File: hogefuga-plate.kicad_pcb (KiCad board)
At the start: 2 copper layers, 95.2 x 76.2 mm, 23 parts

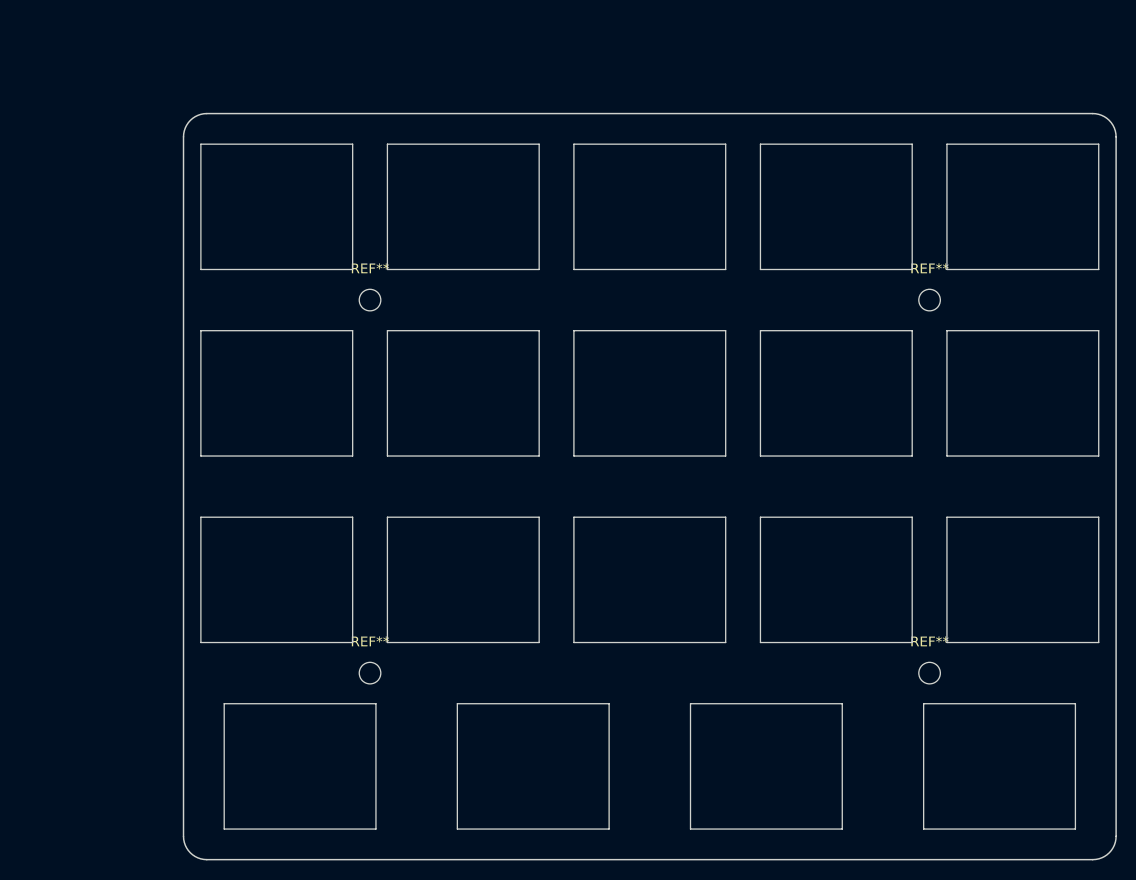
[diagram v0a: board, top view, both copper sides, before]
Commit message: rev0.2
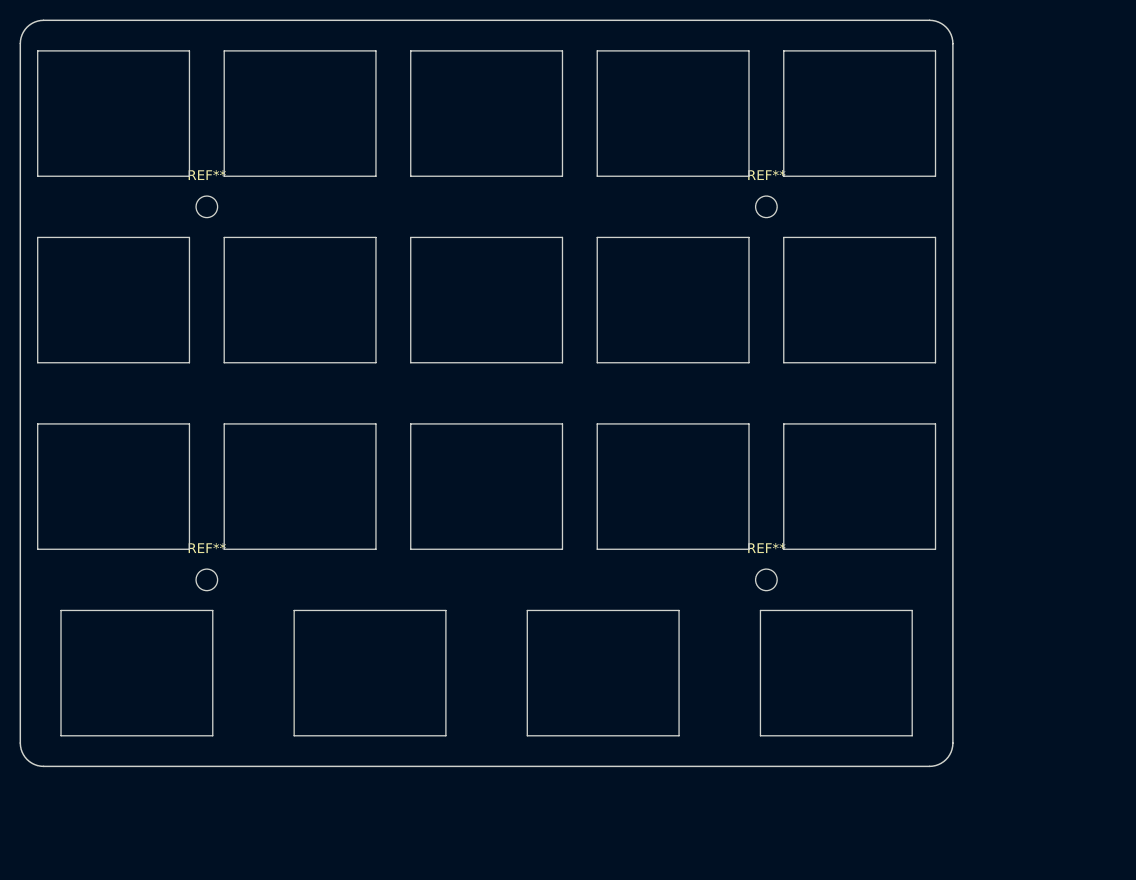
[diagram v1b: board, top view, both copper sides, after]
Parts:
- removed the ALPS_SKCM_CUTOUT at (119.1, 78.6)
- removed the ALPS_SKCM_CUTOUT at (157.2, 116.7)
- removed the ALPS_SKCM_CUTOUT at (81.0, 97.6)
- removed the ALPS_SKCM_CUTOUT at (154.8, 135.7)
- removed the ALPS_SKCM_CUTOUT at (107.2, 135.7)
- removed the ALPS_SKCM_CUTOUT at (138.1, 116.7)
- removed the ALPS_SKCM_CUTOUT at (81.0, 78.6)
- removed the ALPS_SKCM_CUTOUT at (119.1, 116.7)
- removed the ALPS_SKCM_CUTOUT at (81.0, 116.7)
- removed the ALPS_SKCM_CUTOUT at (157.2, 97.6)
- removed the ALPS_SKCM_CUTOUT at (119.1, 97.6)
- removed the ALPS_SKCM_CUTOUT at (100.0, 97.6)
- removed the ALPS_SKCM_CUTOUT at (100.0, 116.7)
- removed the ALPS_SKCM_CUTOUT at (157.2, 78.6)
- removed the ALPS_SKCM_CUTOUT at (131.0, 135.7)
- removed the ALPS_SKCM_CUTOUT at (83.3, 135.7)
- removed the ALPS_SKCM_CUTOUT at (138.1, 78.6)
- removed the ALPS_SKCM_CUTOUT at (100.0, 78.6)
- removed the ALPS_SKCM_CUTOUT at (138.1, 97.6)
- removed the REF** at (90.5, 126.2)
- removed the REF** at (147.6, 88.1)
- removed the REF** at (90.5, 88.1)
- removed the REF** at (147.6, 126.2)
- added ALPS_SKCM_CUTOUT: VAL**, keyboard_parts:ALPS_SKCM_CUTOUT, F.Cu at (140.5, 69.1)
- added ALPS_SKCM_CUTOUT: VAL**, keyboard_parts:ALPS_SKCM_CUTOUT, F.Cu at (64.3, 88.1)
- added ALPS_SKCM_CUTOUT: VAL**, keyboard_parts:ALPS_SKCM_CUTOUT, F.Cu at (64.3, 107.2)
- added ALPS_SKCM_CUTOUT: VAL**, keyboard_parts:ALPS_SKCM_CUTOUT, F.Cu at (83.3, 107.2)
- added ALPS_SKCM_CUTOUT: VAL**, keyboard_parts:ALPS_SKCM_CUTOUT, F.Cu at (102.4, 107.2)
- added ALPS_SKCM_CUTOUT: VAL**, keyboard_parts:ALPS_SKCM_CUTOUT, F.Cu at (121.4, 107.2)
- added ALPS_SKCM_CUTOUT: VAL**, keyboard_parts:ALPS_SKCM_CUTOUT, F.Cu at (140.5, 107.2)
- added ALPS_SKCM_CUTOUT: VAL**, keyboard_parts:ALPS_SKCM_CUTOUT, F.Cu at (138.1, 126.2)
- added ALPS_SKCM_CUTOUT: VAL**, keyboard_parts:ALPS_SKCM_CUTOUT, F.Cu at (114.3, 126.2)
- added ALPS_SKCM_CUTOUT: VAL**, keyboard_parts:ALPS_SKCM_CUTOUT, F.Cu at (90.5, 126.2)
- added ALPS_SKCM_CUTOUT: VAL**, keyboard_parts:ALPS_SKCM_CUTOUT, F.Cu at (66.7, 126.2)
- added ALPS_SKCM_CUTOUT: VAL**, keyboard_parts:ALPS_SKCM_CUTOUT, F.Cu at (121.4, 69.1)
- added ALPS_SKCM_CUTOUT: VAL**, keyboard_parts:ALPS_SKCM_CUTOUT, F.Cu at (102.4, 69.1)
- added ALPS_SKCM_CUTOUT: VAL**, keyboard_parts:ALPS_SKCM_CUTOUT, F.Cu at (83.3, 69.1)
- added ALPS_SKCM_CUTOUT: VAL**, keyboard_parts:ALPS_SKCM_CUTOUT, F.Cu at (64.3, 69.1)
- added ALPS_SKCM_CUTOUT: VAL**, keyboard_parts:ALPS_SKCM_CUTOUT, F.Cu at (140.5, 88.1)
- added ALPS_SKCM_CUTOUT: VAL**, keyboard_parts:ALPS_SKCM_CUTOUT, F.Cu at (121.4, 88.1)
- added ALPS_SKCM_CUTOUT: VAL**, keyboard_parts:ALPS_SKCM_CUTOUT, F.Cu at (102.4, 88.1)
- added ALPS_SKCM_CUTOUT: VAL**, keyboard_parts:ALPS_SKCM_CUTOUT, F.Cu at (83.3, 88.1)
- added REF**: MountingHole_2.2mm_M2, MountingHole:MountingHole_2.2mm_M2, F.Cu at (131.0, 78.6)
- added REF**: MountingHole_2.2mm_M2, MountingHole:MountingHole_2.2mm_M2, F.Cu at (131.0, 116.7)
- added REF**: MountingHole_2.2mm_M2, MountingHole:MountingHole_2.2mm_M2, F.Cu at (73.8, 116.7)
- added REF**: MountingHole_2.2mm_M2, MountingHole:MountingHole_2.2mm_M2, F.Cu at (73.8, 78.6)
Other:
- board size 95.2 x 76.2 mm -> 95.3 x 76.2 mm
